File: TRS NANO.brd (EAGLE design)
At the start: 69.2 x 64.5 mm, 27 parts, among them M1 ARDUINO-NANO-3.0, Q5 BC548, Q6 BC548, Q7 BC548, Q8 BC548, T1 351, T3 351, T41 351, T42 351

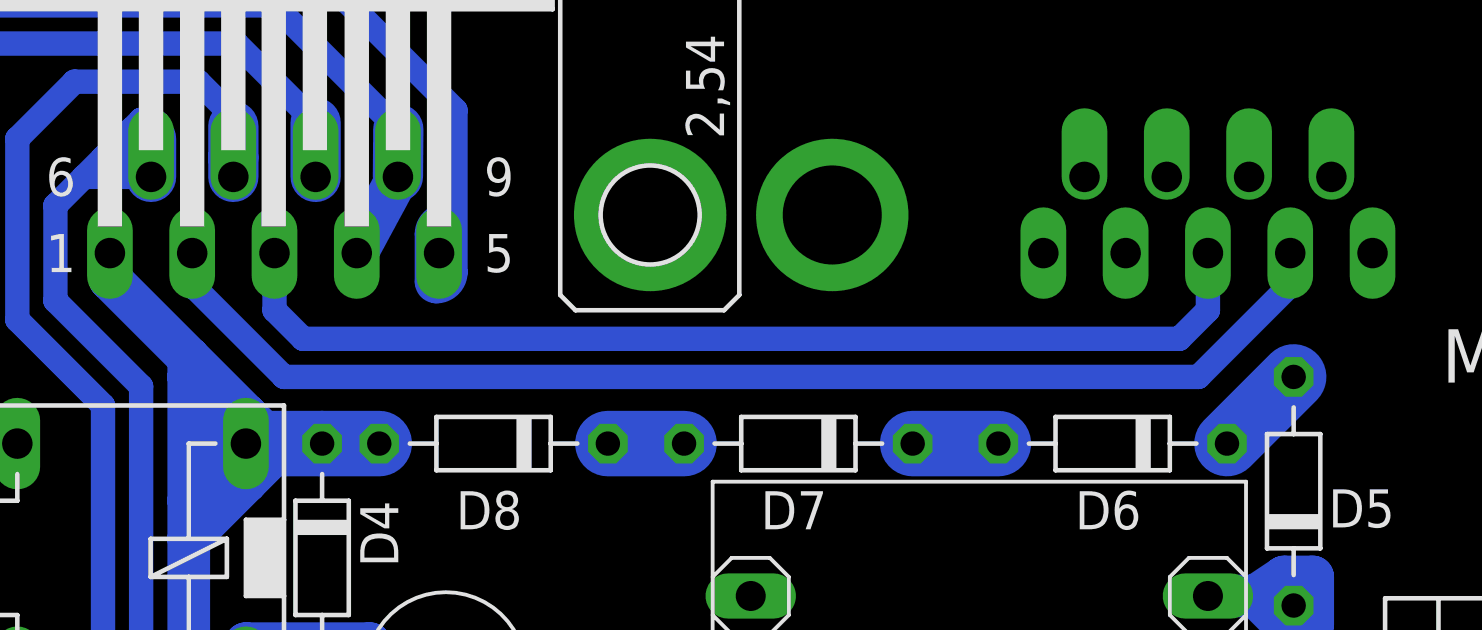
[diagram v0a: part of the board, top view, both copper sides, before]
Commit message: atualiza placa
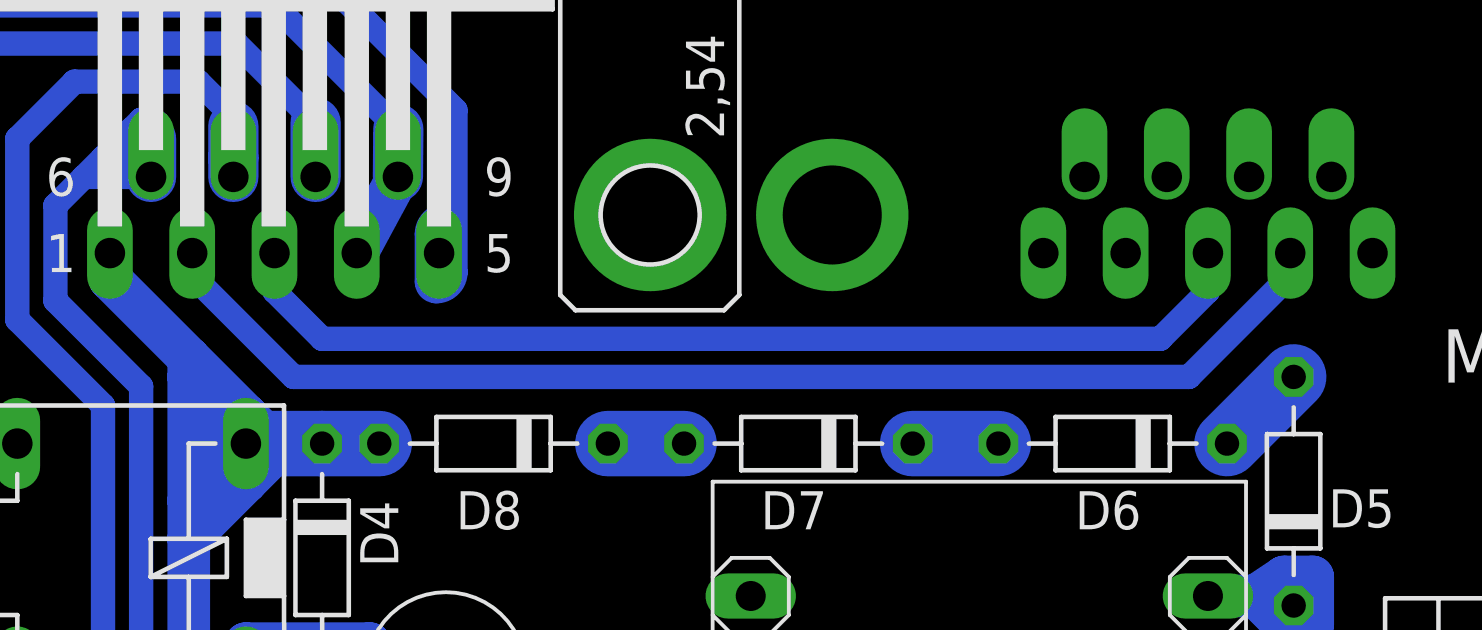
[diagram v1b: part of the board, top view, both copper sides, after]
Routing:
- net TEMP: track 35.7 -> 35.0 mm
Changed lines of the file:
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@@
 <contactref element="FDB9" pad="3"/>
 <contactref element="MDB9" pad="3"/>
-<wire x1="20.955" y1="48.895" x2="50.165" y2="48.895" width="0.8128" layer="16"/>
-<wire x1="50.165" y1="48.895" x2="51.1175" y2="49.8475" width="0.8128" layer="16"/>
-<wire x1="51.1175" y1="49.8475" x2="51.1175" y2="51.7525" width="0.8128" layer="16"/>
-<wire x1="20.0025" y1="51.7525" x2="20.0025" y2="49.8475" width="0.8128" layer="16"/>
-<wire x1="20.0025" y1="49.8475" x2="20.955" y2="48.895" width="0.8128" layer="16"/>
+<wire x1="21.59" y1="48.895" x2="49.53" y2="48.895" width="0.8128" layer="16"/>
+<wire x1="49.53" y1="48.895" x2="51.1175" y2="50.4825" width="0.8128" layer="16"/>
+<wire x1="51.1175" y1="50.4825" x2="51.1175" y2="51.7525" width="0.8128" layer="16"/>
+<wire x1="20.0025" y1="51.7525" x2="20.0025" y2="50.4825" width="0.8128" layer="16"/>
+<wire x1="20.0025" y1="50.4825" x2="21.59" y2="48.895" width="0.8128" layer="16"/>
 </signal>
 <signal name="T41">
@@
 <contactref element="FDB9" pad="2"/>
 <contactref element="MDB9" pad="2"/>
-<wire x1="17.2593" y1="51.7525" x2="17.2593" y2="50.6857" width="0.8128" layer="16"/>
-<wire x1="17.2593" y1="50.6857" x2="20.32" y2="47.625" width="0.8128" layer="16"/>
-<wire x1="20.32" y1="47.625" x2="50.8" y2="47.625" width="0.8128" layer="16"/>
-<wire x1="53.8607" y1="51.7525" x2="53.8607" y2="50.6857" width="0.8128" layer="16"/>
-<wire x1="53.8607" y1="50.6857" x2="50.8" y2="47.625" width="0.8128" layer="16"/>
+<wire x1="17.2593" y1="51.7525" x2="17.2593" y2="51.0032" width="0.8128" layer="16"/>
+<wire x1="17.2593" y1="51.0032" x2="20.6375" y2="47.625" width="0.8128" layer="16"/>
+<wire x1="20.6375" y1="47.625" x2="50.4825" y2="47.625" width="0.8128" layer="16"/>
+<wire x1="53.8607" y1="51.7525" x2="53.8607" y2="51.0032" width="0.8128" layer="16"/>
+<wire x1="53.8607" y1="51.0032" x2="50.4825" y2="47.625" width="0.8128" layer="16"/>
 </signal>
 <signal name="N$10">
